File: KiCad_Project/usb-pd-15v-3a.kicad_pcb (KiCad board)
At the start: 2 copper layers, 59.1 x 99.1 mm, 55 parts, among them J1 Conn_01x02_Male, J10 2.5mm/5.5mm (PC-G2.5-PCB), J11 Conn_01x02_Male, J12 Conn_01x02_Male, J13 Conn_01x02_Male, J14 ETB11040B000Z, J15 Conn_01x02_Male, J16 Conn_01x02_Male, J17 Conn_01x02_Male, J2 Conn_01x02_Male, J3 Conn_01x02_Male, J4 Conn_01x02_Male, J5 Conn_01x02_Male, J6 Conn_01x02_Male, J7 Conn_01x02_Male, J8 Conn_01x02_Male, J9 Conn_02x08_Odd_Even, U1 LM340S-12/NOPB, U2 L4940D2T5-DR, U3 LM2596S-12

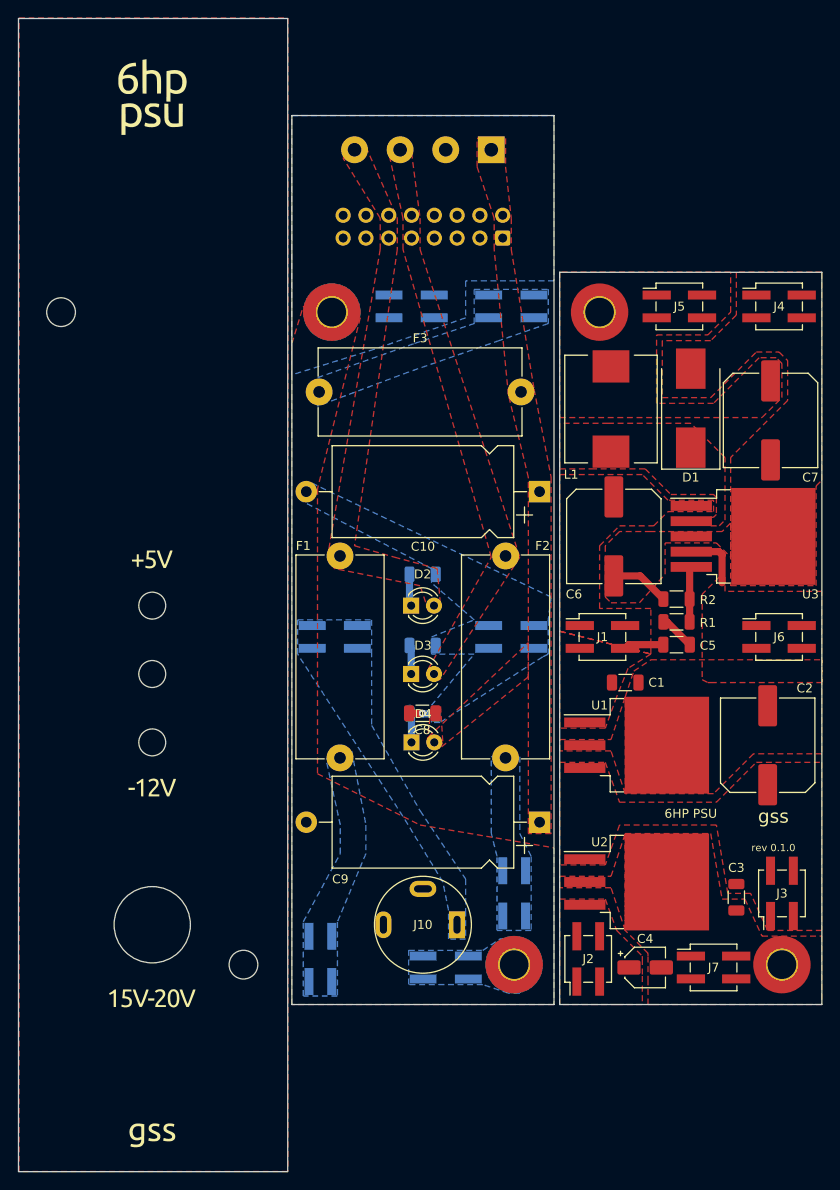
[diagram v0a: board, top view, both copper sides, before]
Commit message: update psu git
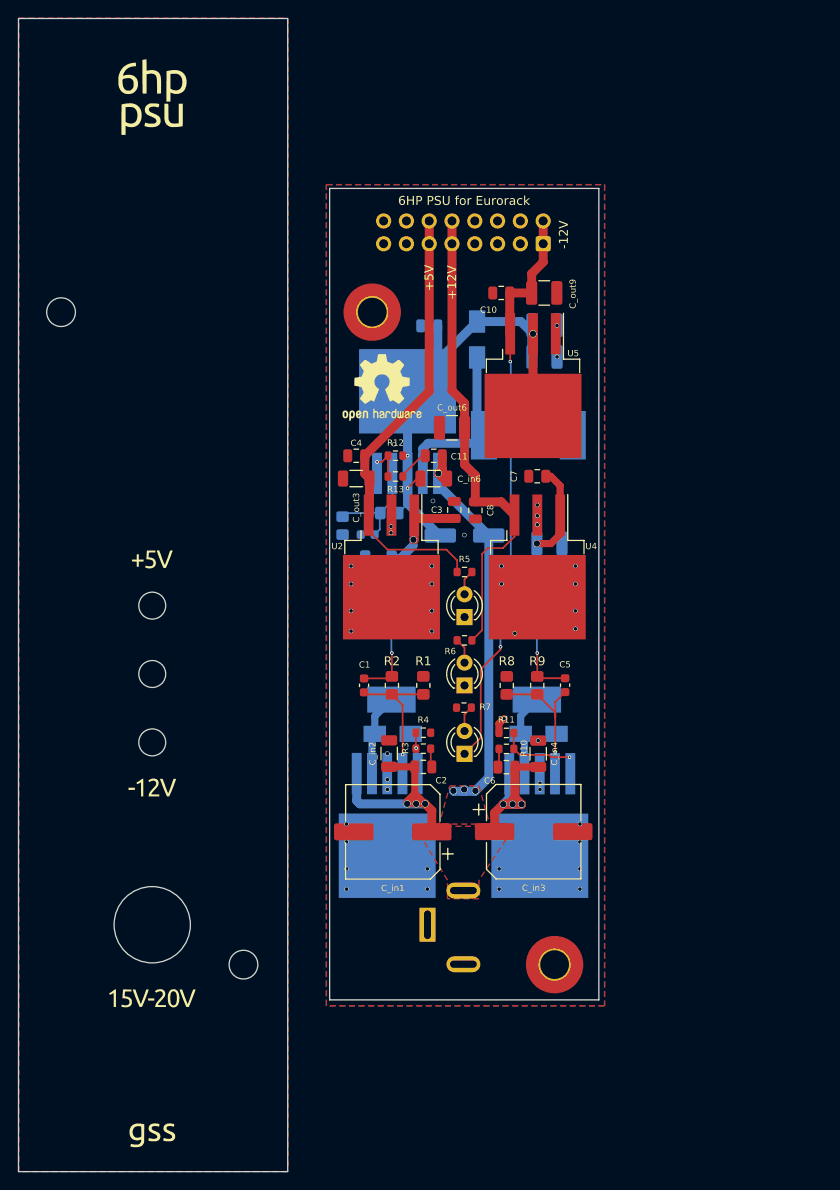
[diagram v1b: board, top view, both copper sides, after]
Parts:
- removed F1, F2, F3: Fuse_Small, Fuse:Fuseholder_Cylinder-5x20mm_Schurter_0031_8201_Horizontal_Open
- removed H3, H4: MountingHole_Pad, MountingHole:MountingHole_3.2mm_M3_Pad_TopBottom
- removed J10: 2.5mm/5.5mm (PC-G2.5-PCB), OS_Connectors:DC-Barrel_2.5mm_5.5mm_Vertical
- removed J11, J12, J13, J15, J16, J17, J8: Conn_01x02_Male, Connector_PinSocket_2.54mm:PinSocket_2x02_P2.54mm_Vertical_SMD
- removed J14: ETB11040B000Z, TerminalBlock:TerminalBlock_bornier-4_P5.08mm
- removed J3, J4, J5, J6, J7: Conn_01x02_Male, Connector_PinHeader_2.54mm:PinHeader_2x02_P2.54mm_Vertical_SMD
- removed J9: Conn_02x08_Odd_Even, Connector_IDC:IDC-Header_2x08_P2.54mm_Vertical
- added C11: 100nF, Capacitor_SMD:C_0805_2012Metric, F.Cu at (29.5, 45.2)
- added C12: 22n, Capacitor_SMD:C_0603_1608Metric, B.Cu at (22.1, 54.0)
- added C_in1: 220uF, Capacitor_SMD:CP_Elec_10x7.7, F.Cu at (24.9, 87.1)
- added C_in2: 100nF, Capacitor_SMD:C_1206_3216Metric, F.Cu at (24.5, 78.4)
- added C_in3: 220uF, Capacitor_SMD:CP_Elec_10x7.7, F.Cu at (40.6, 87.1)
- added C_in4: 100nF, Capacitor_SMD:C_1206_3216Metric, F.Cu at (41.1, 78.4)
- added C_in5: 100uF, Capacitor_SMD:CP_Elec_6.3x7.7, B.Cu at (32.9, 54.1)
- added C_in6: 100nF, Capacitor_SMD:C_1206_3216Metric, F.Cu at (29.5, 47.8)
- added C_out1: 47u, Capacitor_SMD:C_1206_3216Metric, B.Cu at (23.3, 59.2)
- added C_out2: 47u, Capacitor_SMD:C_1206_3216Metric, B.Cu at (23.3, 56.6)
- added C_out3: 47u, Capacitor_SMD:C_1206_3216Metric, F.Cu at (20.8, 47.8)
- added C_out4: 100uF, Inductor_SMD:L_1210_3225Metric, B.Cu at (42.4, 58.5)
- added C_out5: 100uF, Inductor_SMD:L_1210_3225Metric, B.Cu at (42.4, 55.0)
- added C_out6: 100uF, Inductor_SMD:L_1210_3225Metric, F.Cu at (31.5, 42.1)
- added C_out7: 100uF, Inductor_SMD:L_1210_3225Metric, B.Cu at (41.8, 34.2)
- added C_out8: 100uF, Inductor_SMD:L_1210_3225Metric, B.Cu at (41.8, 30.7)
- added C_out9: 100uF, Inductor_SMD:L_1210_3225Metric, F.Cu at (41.8, 27.1)
- added D5: SS54, Diode_SMD:D_SMA, B.Cu at (41.1, 76.2)
- added D6: SS54, Diode_SMD:D_SMA, B.Cu at (34.3, 32.3)
- added L2: 33uH, Inductor_SMD:L_12x12mm_H8mm, B.Cu at (41.0, 67.4)
- added L3: 33uH, Inductor_SMD:L_12x12mm_H8mm, B.Cu at (40.0, 42.9)
- added R10: 47k, Resistor_SMD:R_0603_1608Metric, F.Cu at (37.6, 77.9)
- added R11: 47k, Resistor_SMD:R_0603_1608Metric, F.Cu at (37.6, 76.1)
- added R12: 47k, Resistor_SMD:R_0603_1608Metric, F.Cu at (25.2, 45.2)
- added R13: 47k, Resistor_SMD:R_0603_1608Metric, F.Cu at (25.2, 47.5)
- added R14: 15k, Resistor_SMD:R_0805_2012Metric_Pad1.20x1.40mm_HandSolder, B.Cu at (19.3, 53.0)
- added R15: 1k2, Resistor_SMD:R_0805_2012Metric_Pad1.20x1.40mm_HandSolder, B.Cu at (24.5, 51.6)
- added R6: 8k2, Resistor_SMD:R_0603_1608Metric, F.Cu at (32.9, 65.8)
- added R7: 8k2, Resistor_SMD:R_0603_1608Metric, F.Cu at (32.8, 73.3)
- added R8: 1k2, Resistor_SMD:R_0805_2012Metric_Pad1.20x1.40mm_HandSolder, F.Cu at (37.6, 70.8)
- added R9: 15k, Resistor_SMD:R_0805_2012Metric_Pad1.20x1.40mm_HandSolder, F.Cu at (41.0, 70.8)
- added REF**: OSHW-Logo2_9.8x8mm_SilkScreen, Symbol:OSHW-Logo2_9.8x8mm_SilkScreen, F.Cu at (23.7, 37.6)
- added REF**: OSHW-Logo2_9.8x8mm_SilkScreen, Symbol:OSHW-Logo2_9.8x8mm_SilkScreen, B.Cu at (23.4, 101.3)
- added U4: L7812, Package_TO_SOT_SMD:TO-263-3_TabPin2, F.Cu at (41.0, 57.6)
- added U5: L7912, Package_TO_SOT_SMD:TO-263-3_TabPin2, F.Cu at (40.5, 37.4)
- added U6: LM2596S-ADJ, Package_TO_SOT_SMD:TO-263-5_TabPin3, B.Cu at (26.5, 41.4)
- C1: value 100n -> 47n; footprint Capacitor_SMD:C_1206_3216Metric -> Capacitor_SMD:C_0603_1608Metric
- C10: value 470uF/radial/25V -> 100nF; footprint Capacitor_THT:CP_Axial_L20.0mm_D10.0mm_P26.00mm_Horizontal -> Capacitor_SMD:C_0805_2012Metric
- C2, C6: value 100uF/50V/Low ESR -> 100nF; footprint Capacitor_SMD:C_Elec_10x10.2 -> Capacitor_SMD:C_0805_2012Metric
- C3, C8: value 100n -> 100nF; footprint Capacitor_SMD:C_1206_3216Metric -> Capacitor_SMD:C_0805_2012Metric
- C4: value 22uF/10V/Low ESR -> 100nF; footprint Capacitor_SMD:CP_Elec_4x5.8 -> Capacitor_SMD:C_0805_2012Metric
- C5: value C_Small -> 22n; footprint Capacitor_SMD:C_1206_3216Metric -> Capacitor_SMD:C_0603_1608Metric
- C7: value 330uF/25V/Low ESR -> 100nF; footprint Capacitor_SMD:C_Elec_10x10.2 -> Capacitor_SMD:C_0805_2012Metric
- C9: value 470uF/radial/25V -> 100nF; footprint Capacitor_THT:CP_Axial_L20.0mm_D10.0mm_P26.00mm_Horizontal -> Capacitor_SMD:C_0805_2012Metric; moved to B.Cu
- D1: value B540C-13-F -> SS54; footprint Diode_SMD:D_SMC_Handsoldering -> Diode_SMD:D_SMA; moved to B.Cu
- D2: value yellow -> (none)
- D3: value red -> (none)
- D4: value blue -> (none)
- J1: value Conn_01x02_Male -> 2.5mm/5.5mm (PC-G2.5-PCB); footprint Connector_PinHeader_2.54mm:PinHeader_2x02_P2.54mm_Vertical_SMD -> Connectors:DC_Barrel_Jack_2.5mm_5.7mm_Verrtical
- J2: value Conn_01x02_Male -> Conn_02x08_Odd_Even; footprint Connector_PinHeader_2.54mm:PinHeader_2x02_P2.54mm_Vertical_SMD -> Connector_IDC:IDC-Header_2x08_P2.54mm_Vertical; moved to B.Cu
- L1: value 33uH/ETQP4M330KVC -> 33uH; footprint Inductor_SMD:L_Neosid_SM-PIC1004H -> Inductor_SMD:L_12x12mm_H8mm; moved to B.Cu
- R1: value R -> 1k2; footprint Resistor_SMD:R_1206_3216Metric -> Resistor_SMD:R_0805_2012Metric_Pad1.20x1.40mm_HandSolder
- R2: value R -> 6k2; footprint Resistor_SMD:R_1206_3216Metric -> Resistor_SMD:R_0805_2012Metric_Pad1.20x1.40mm_HandSolder
- R3, R4: value R -> 47k; footprint Resistor_SMD:R_1206_3216Metric -> Resistor_SMD:R_0603_1608Metric; moved to F.Cu
- R5: value R -> 2k2; footprint Resistor_SMD:R_1206_3216Metric -> Resistor_SMD:R_0603_1608Metric; moved to F.Cu
- U1: value LM340S-12/NOPB -> LM2596S-ADJ; footprint Package_TO_SOT_SMD:TO-263-3_TabPin2 -> Package_TO_SOT_SMD:TO-263-5_TabPin3; moved to B.Cu
- U2: value L4940D2T5-DR -> L7805
- U3: value LM2596S-12 -> LM2596S-ADJ; moved to B.Cu
- moved J2 79.9 mm to (41.7, 21.6)
- moved C4 65.5 mm to (20.8, 45.2), turned to 180 degrees
- moved C9 56.7 mm to (29.0, 30.7)
- moved C3 53.4 mm to (31.8, 51.2), turned to -90 degrees
- moved D1 49.2 mm to (24.9, 76.2), turned to 0 degrees
- moved U2 44.5 mm to (24.7, 57.6), turned to -90 degrees
- moved U3 39.4 mm to (41.3, 86.4), turned to -90 degrees
- moved C2 38.5 mm to (28.3, 79.9), turned to 0 degrees
- moved L1 36.8 mm to (24.7, 67.4)
- moved J1 35.6 mm to (32.8, 97.5), turned to -90 degrees
- moved R2 33.1 mm to (24.8, 70.8), turned to 90 degrees
- moved U1 29.2 mm to (24.3, 86.4), turned to -90 degrees
- moved C1 29.1 mm to (21.7, 70.8), turned to -90 degrees
- moved R1 29.1 mm to (28.3, 70.8), turned to 90 degrees
- moved C6 28.4 mm to (37.6, 79.9), turned to 180 degrees
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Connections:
- C1 pad 1: /main_psu/GND2 -> Net-(C1-Pad1)
- C1 pad 2: /main_psu/+15V -> Net-(C1-Pad2)
- C10 pad 1: -12V_Eurorack -> GND
- C10 pad 2: GND -> -12V
- C2 pad 1: /main_psu/+12V -> Vin
- C2 pad 2: /main_psu/GND2 -> Net-(C2-Pad2)
- C3 pad 1: /main_psu/GND3 -> GND
- C3 pad 2: /main_psu/+12V -> Net-(C1-Pad1)
- C4 pad 1: /main_psu/+5V -> +5V
- C4 pad 2: /main_psu/GND3 -> GND
- C5 pad 1: /main_psu/+15V -> Net-(C5-Pad1)
- C6 pad 1: /main_psu/+15V -> Vin
- C6 pad 2: /main_psu/-12V -> Net-(C6-Pad2)
- C7 pad 1: /main_psu/GND1 -> GND
- C7 pad 2: /main_psu/-12V -> Net-(C5-Pad1)
- C8 pad 1: -12V_Eurorack -> +12V
- C9 pad 1: -12V_Eurorack -> -14.5V
- D1 pad 2: /main_psu/-12V -> GND
- D2 pad 1: Net-(D2-Pad1) -> GND
- D2 pad 2: 5V_Eurorack -> Net-(D2-Pad2)
- D3 pad 1: Net-(D3-Pad1) -> GND
- D3 pad 2: 12V_Eurorack -> Net-(D3-Pad2)
- D4 pad 1: Net-(D4-Pad1) -> -12V
- D4 pad 2: -12V_Eurorack -> Net-(D4-Pad2)
- H1 pad 1: /main_psu/GND1 -> GND
- H2 pad 1: /main_psu/GND3 -> GND
- J1 pad 1: /main_psu/+15V -> GND
- J1 pad 2: /main_psu/+15V -> Vin
- J1 pad 3: /main_psu/+15V -> unconnected-(J1-Pad3)
- J2 pad 1: /main_psu/+5V -> -12V
- J2 pad 2: /main_psu/+5V -> -12V
- J2 pad 3: /main_psu/+5V -> GND
- J2 pad 4: /main_psu/+5V -> GND
- L1 pad 2: /main_psu/GND1 -> Net-(C1-Pad1)
- R1 pad 1: Net-(C5-Pad2) -> Net-(C1-Pad2)
- R1 pad 2: Net-(R1-Pad2) -> GND
- R2 pad 1: /main_psu/-12V -> Net-(C1-Pad2)
- R2 pad 2: Net-(R1-Pad2) -> Net-(C1-Pad1)
- R3 pad 1: Net-(D2-Pad1) -> Net-(C2-Pad2)
- R3 pad 2: GND -> Net-(R3-Pad2)
- R4 pad 1: Net-(D3-Pad1) -> Net-(R3-Pad2)
- R5 pad 1: Net-(D4-Pad1) -> +5V
- R5 pad 2: GND -> Net-(D2-Pad2)
- U1 pad 1: /main_psu/+15V -> Vin
- U1 pad 2: /main_psu/GND2 -> Net-(D1-Pad1)
- U1 pad 3: /main_psu/+12V -> GND
- U2 pad 1: /main_psu/+12V -> Net-(C1-Pad1)
- U2 pad 2: /main_psu/GND3 -> GND
- U2 pad 3: /main_psu/+5V -> +5V
- U3 pad 1: /main_psu/+15V -> Vin
- U3 pad 2: Net-(D1-Pad1) -> Net-(D5-Pad1)
- U3 pad 3: /main_psu/-12V -> GND
- U3 pad 4: /main_psu/GND2 -> Net-(C5-Pad2)
- U3 pad 5: Net-(R1-Pad2) -> Net-(R10-Pad2)
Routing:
- net Vin: track 0.00 -> 92.3 mm, vias 0 -> 10
- net -12V: track 0.00 -> 64.5 mm, vias 0 -> 2
- net -14.5V: track 0.00 -> 61.6 mm, vias 0 -> 3
- net +12V: track 0.00 -> 54.3 mm
- net +5V: track 0.00 -> 50.3 mm
- net Net-(C5-Pad1): track 0.00 -> 28.5 mm, vias 0 -> 2
- net Net-(C1-Pad1): track 0.00 -> 27.5 mm, vias 0 -> 2
- net Net-(D6-Pad1): track 0.00 -> 19.2 mm
- net Net-(C1-Pad2): track 0.00 -> 16.2 mm, vias 0 -> 1
- net Net-(C5-Pad2): track 3.99 -> 16.3 mm, vias 0 -> 1
- net Net-(C12-Pad2): track 0.00 -> 12.0 mm
- net Net-(R10-Pad2): track 0.00 -> 10.2 mm, vias 0 -> 1
- net Net-(D5-Pad1): track 0.00 -> 9.18 mm
- net Net-(D1-Pad1): track 0.00 -> 9.14 mm
- net /main_psu/GND2: track 6.71 -> 0.00 mm
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- added copper zone on In1.Cu, net GND
- added copper zone on In2.Cu, net GND
- added copper zone on F.Cu, net Vin
- removed copper zone on F.Cu, net -12V_Eurorack
- removed copper zone on B.Cu, net /interface/+12V
- removed copper zone on B.Cu, net /interface/+15V
- removed copper zone on B.Cu, net /interface/+5V
- removed copper zone on B.Cu, net /interface/-12V
- removed copper zone on F.Cu, net /main_psu/+12V
- removed copper zone on F.Cu, net /main_psu/+15V
- removed copper zone on F.Cu, net /main_psu/+5V
- removed copper zone on F.Cu, net /main_psu/-12V
- removed copper zone on F.Cu, net /main_psu/GND1
- removed copper zone on F.Cu, net /main_psu/GND2
- removed copper zone on F.Cu, net /main_psu/GND3
- removed copper zone on F.Cu, net 12V_Eurorack
- removed copper zone on F.Cu, net 5V_Eurorack
- removed copper zone on F.Cu, net Net-(D1-Pad1)
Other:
- board size 59.1 x 99.1 mm -> 30 x 128.5 mm
- copper layers 2 -> 4
- board text added: "+12V"
- board text added: "+5V"
- board text added: "-12V"
- board text added: "15V to 20V"
- board text added: "6HP PSU for Eurorack"
- board text added: "Max Genson Feb 2023"
- board text added: "rev.2"
- board text removed: "6HP PSU"
- board text removed: "gss"
- board text removed: "rev 0.1.0"
